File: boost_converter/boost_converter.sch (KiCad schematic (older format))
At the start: 34 parts, among them J1 Battery +, J2 GND, Q1 N Channel, Q2 N Channel, Q3 N Channel, U1 LM5122

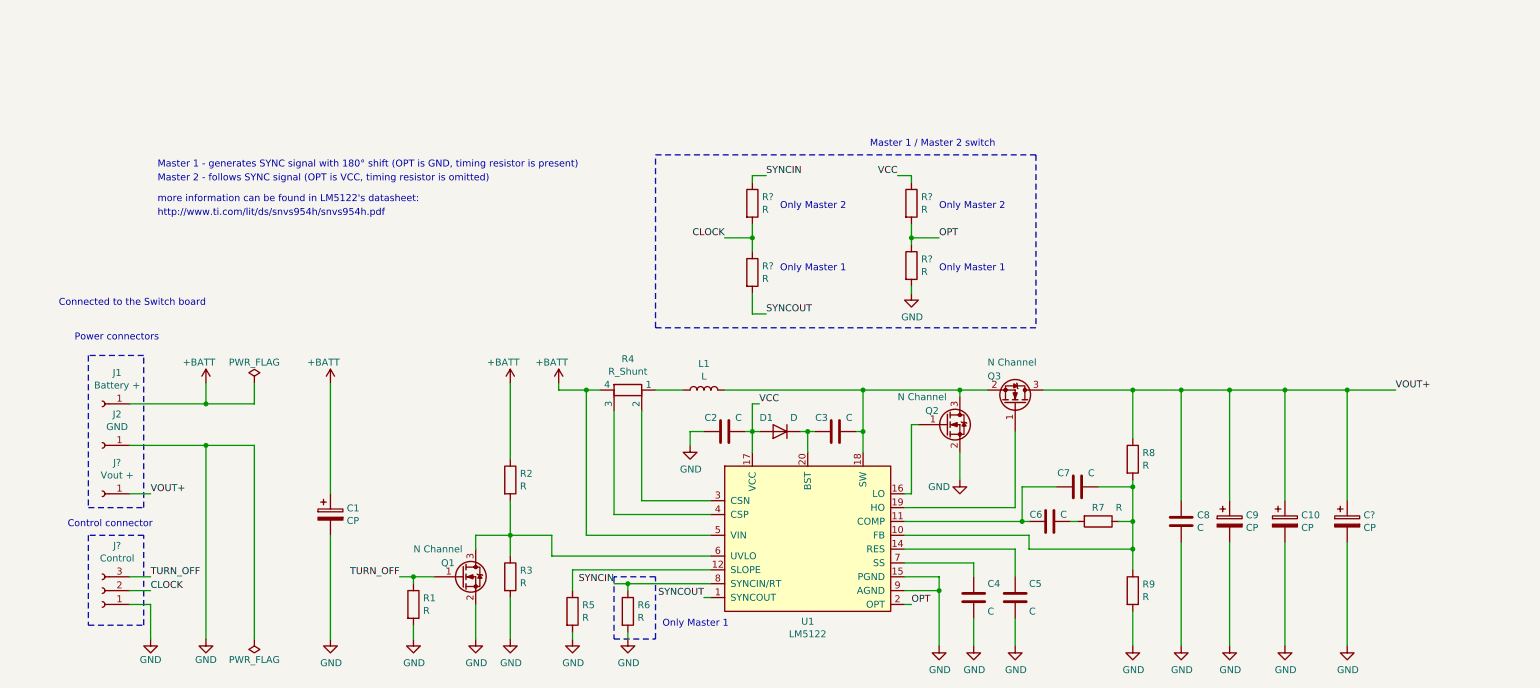
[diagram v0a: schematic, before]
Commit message: started finding components
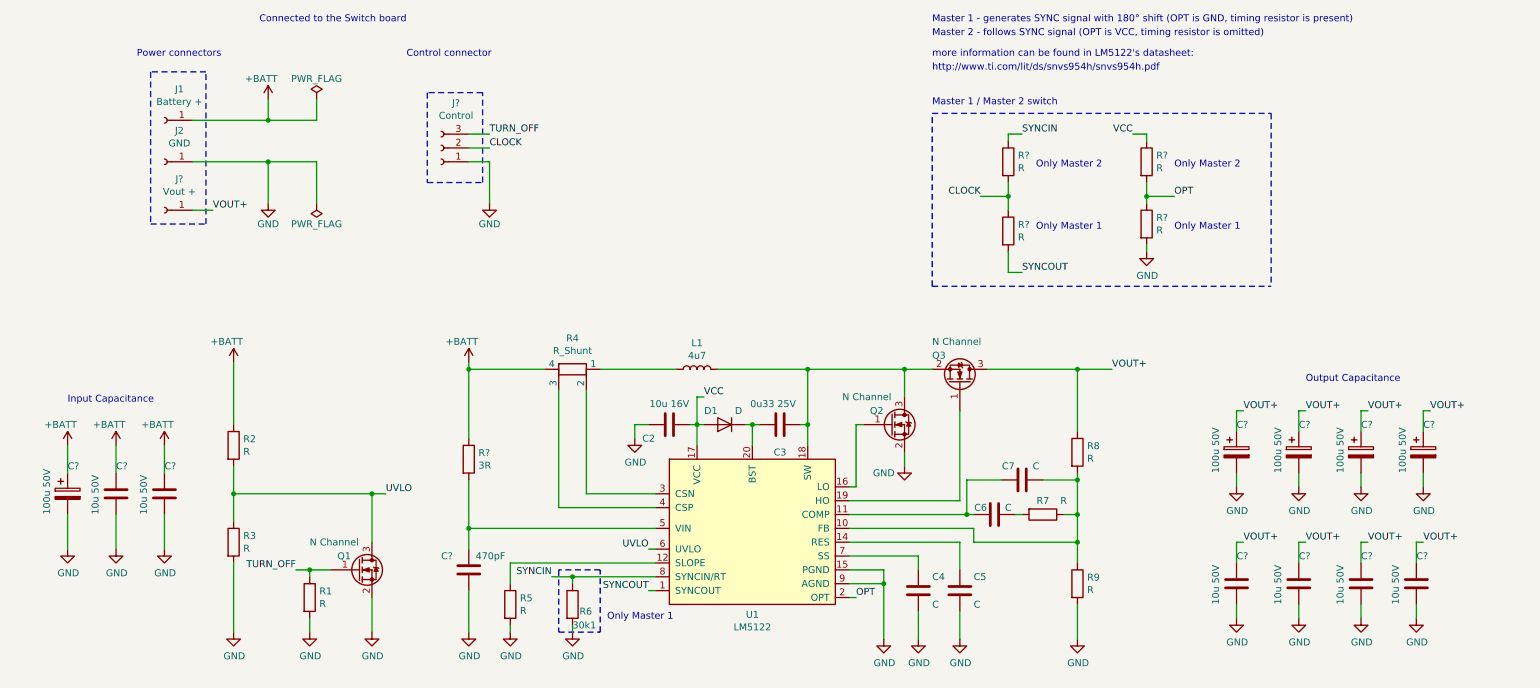
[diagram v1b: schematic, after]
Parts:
- removed C1, C10, C9, C?: CP, symbol Device:CP
- removed C8: C, symbol Device:C
- added C? (x5): 100u 50V, Capacitors_THT:CP_Radial_D10.0mm_P5.00mm, symbol Device:CP
- added C? (x6): 10u 50V, Capacitors_SMD:C_1206, symbol Device:C
- added C?: 470pF, Capacitors_SMD:C_0402, symbol Device:C
- added R?: 3R, Resistors_SMD:R_0402, symbol Device:R
- C2: value C -> 10u 16V; footprint (none) -> Capacitors_SMD:C_0805; MPN (none) -> C2012X5R1C106M085AC
- C3: value C -> 0u33 25V; footprint (none) -> Capacitors_SMD:C_0603; MPN (none) -> 885012206074
- L1: value L -> 4u7; MPN (none) -> SRP1770TA-4R7M
- R6: value R -> 30k1; footprint (none) -> Capacitors_SMD:C_0402; MPN (none) -> CRCW040230K1FKED
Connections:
- net +BATT: now also C?.1, C?.1, C?.1, R?.1; no longer U1.5 (VIN)
- net GND: now also C?.2, C?.2, C?.2, C?.2, C?.2, C?.2, C?.2, C?.2, C?.2, C?.2, C?.2, C?.2
- net VOUT+: now also C?.1, C?.1, C?.1, C?.1, C?.1, C?.1, C?.1, C?.1
- net UVLO: now reaches Q1.3 (D), R2.2, R3.1, U1.6 (UVLO)
- new net: C?.1, R?.2, U1.5 (VIN)
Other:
- note added: "Input Capacitance"
- note added: "Output Capacitance"
- moved on the sheet: C2, C3, C4, C5, C6, C7, D1, J1, J2, J?, L1, Q1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
